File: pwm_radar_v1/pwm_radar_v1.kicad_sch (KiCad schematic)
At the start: 22 parts, among them J1 Conn_Coaxial, J2 Conn_01x01_Pin, J3 Conn_01x01_Pin, J4 Conn_Coaxial, J5 Conn_Coaxial, J6 Conn_Coaxial, J7 Conn_01x01_Pin, J8 Conn_01x01_Pin

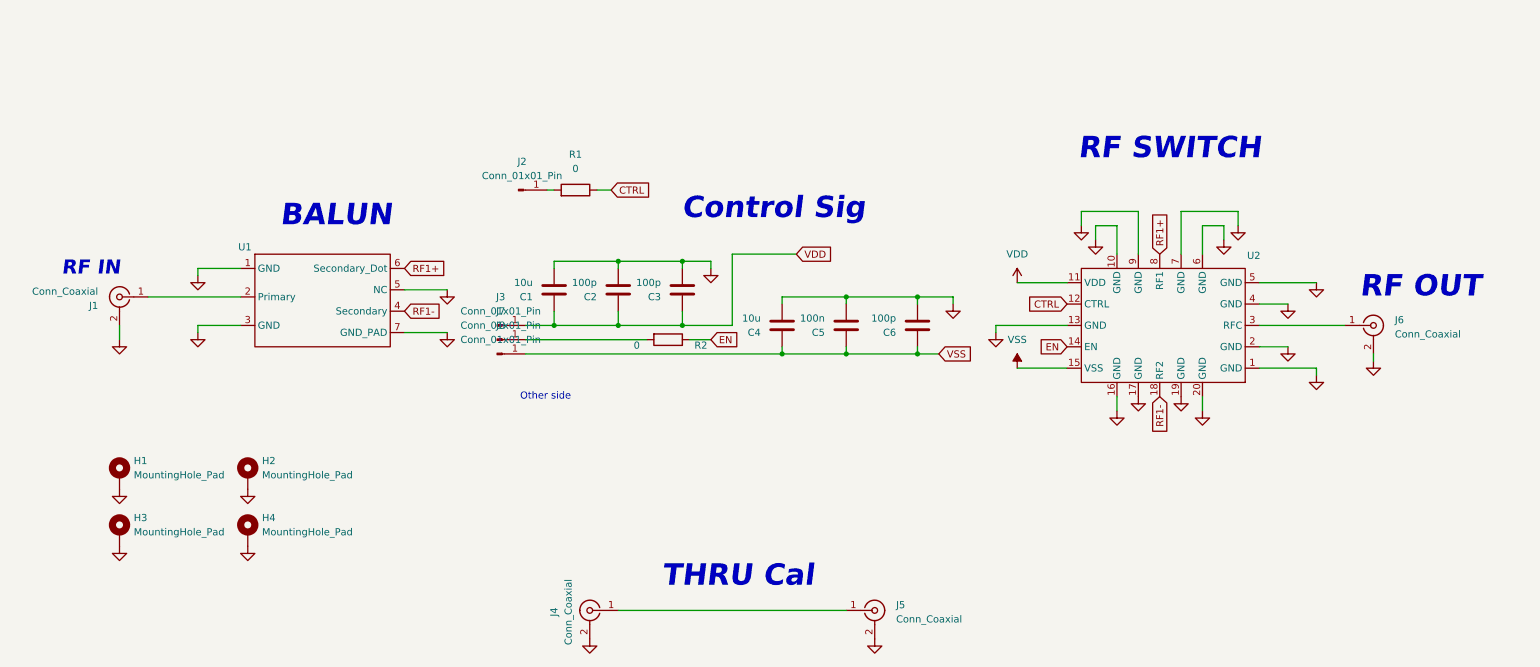
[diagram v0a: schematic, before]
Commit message: changes
changes
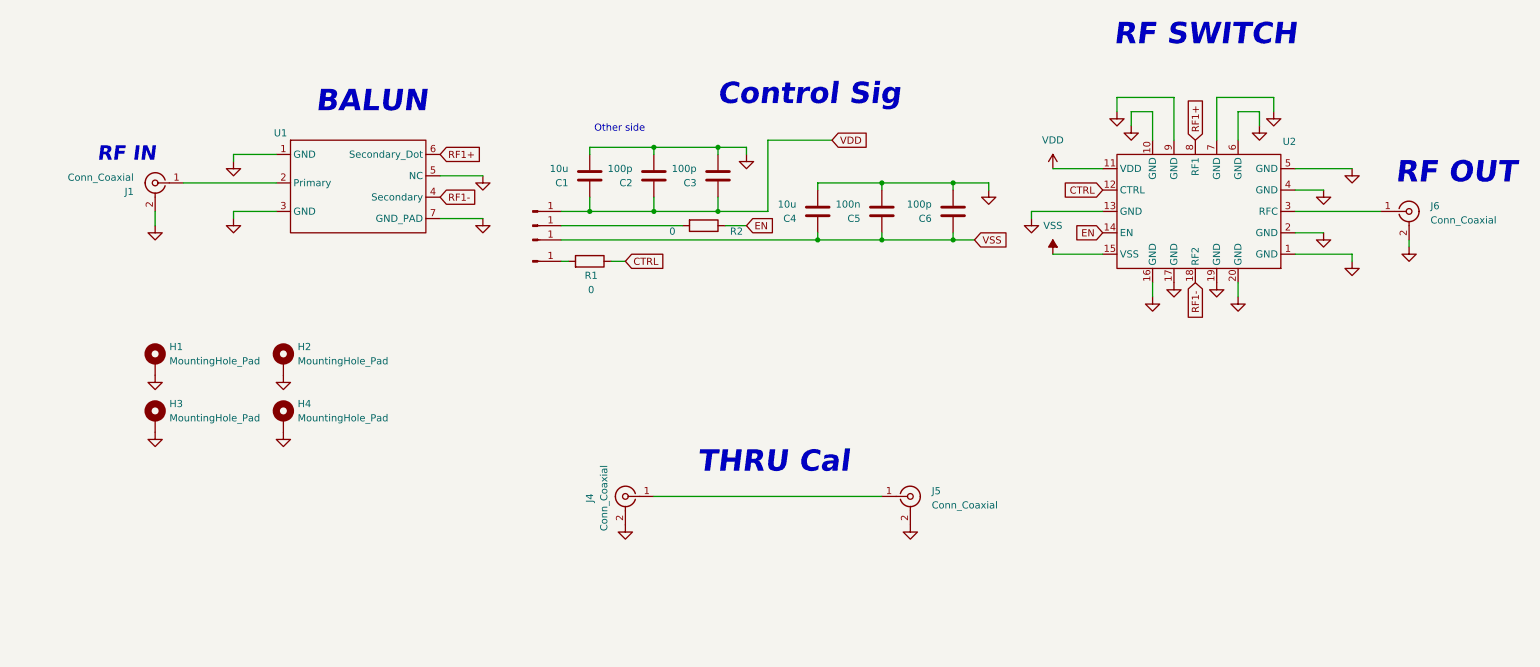
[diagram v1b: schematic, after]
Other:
- company: Center for Non Destructive Evaluation -> (none)
- title: PWM Phased Array Radar -> (none)
- moved on the sheet: C1, C2, C3, C4, C5, C6, H1, H2, H3, H4, J1, J4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
